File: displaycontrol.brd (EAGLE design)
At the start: 77.6 x 58.7 mm, 49 parts, among them IC1 25LC080SN, J1 GRPB052VWQS-RC, J2 5.5x2.1mm Barrel, J3 98424-F52, Q1 MMPQ3904, U1 LPC1315FBD48,551, U2 ADP3300ARTZ-3.3RL7, U3 UDN2987LWTR-6-T, U4 UDN2987LWTR-6-T, Y1 12MHz

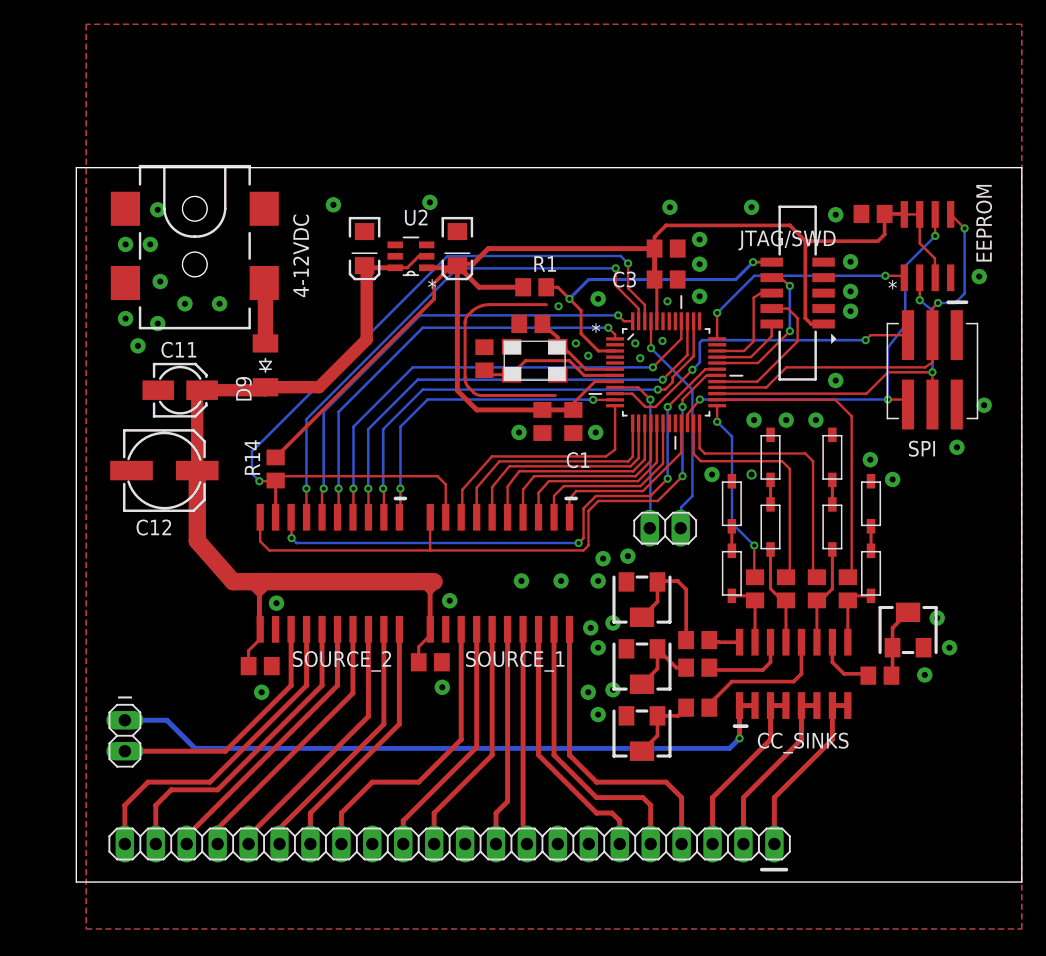
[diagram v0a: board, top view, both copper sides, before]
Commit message: changed trans
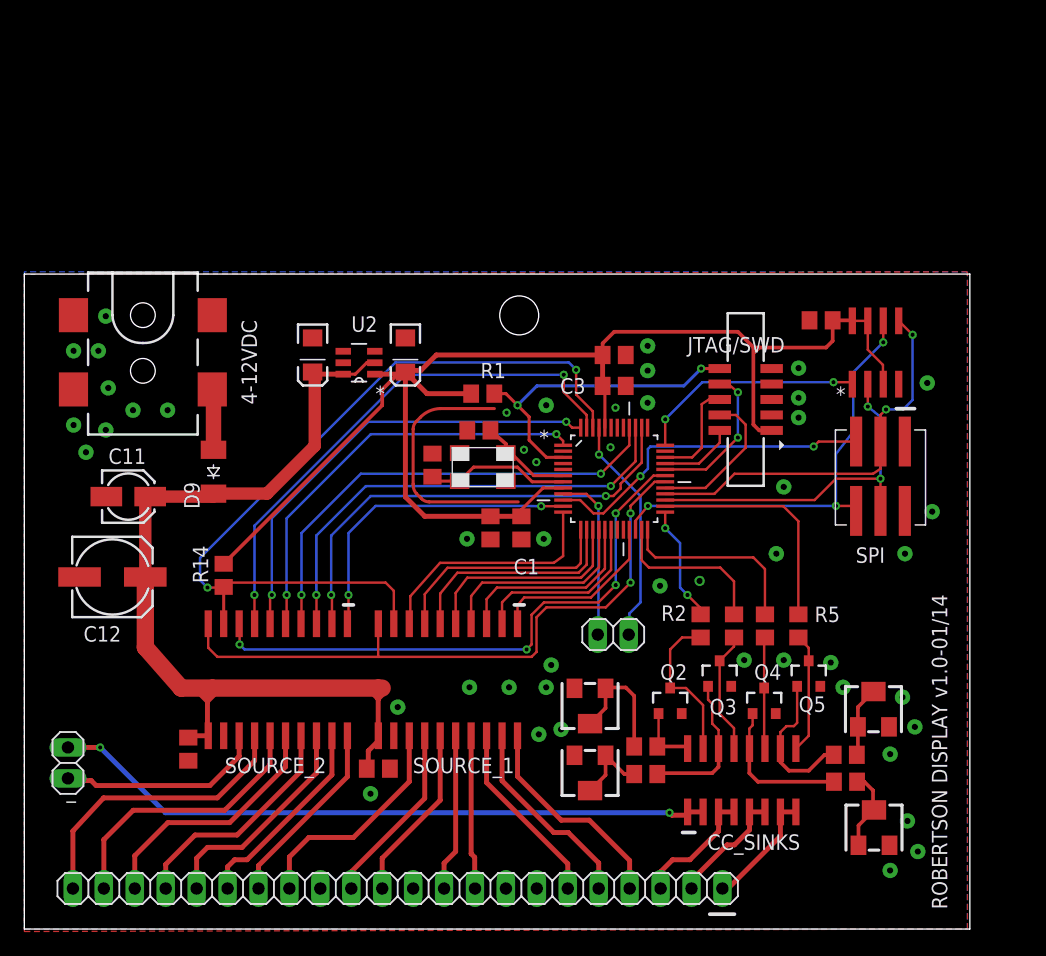
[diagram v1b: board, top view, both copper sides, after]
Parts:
- removed D1, D2, D3, D4, D5, D6, D7, D8: MMSD4148, adafruit:SOD-123
- added Q2, Q3, Q4, Q5: MMBT3904, SparkFun-DiscreteSemi:SOT23-3
- R2, R3, R4, R5: value 4.7k -> 2.7k
- R6, R7, R8, R9: value 14 -> 10
- moved R11 20.6 mm to (69.8, 8.33), turned to 0 degrees
- moved R8 13.6 mm to (67.4, 12.1), turned to 0 degrees
- moved C5 9.72 mm to (37.3, 41.0)
- moved C7 9.72 mm to (23.7, 47.1)
- moved C8 9.72 mm to (31.3, 47.1)
- moved IC1 9.72 mm to (69.9, 47.3)
- moved J3 9.72 mm to (70.3, 37.2)
- moved R6 9.72 mm to (51.0, 15.0)
- moved R7 9.72 mm to (51.0, 12.7)
- moved U4 9.72 mm to (34.8, 20.5)
- moved C11 9.72 mm to (8.53, 35.5)
- moved J2 9.72 mm to (9.73, 50.4)
- moved R14 9.72 mm to (16.4, 29.0)
- moved U2 9.72 mm to (27.5, 46.5)
- moved U3 9.72 mm to (20.8, 20.5)
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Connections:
- removed net N$10: Q1.16, R6.1
- removed net N$11: D5.A, Q1.11, R4.2
- removed net N$12: D5.C, D6.A
- removed net N$14: D7.A, Q1.9, R5.2
- removed net N$15: D7.C, D8.A
- removed net N$17: Q1.14, R7.1
- removed net N$19: Q1.12, R8.1
- removed net N$21: Q1.10, R9.1
- removed net N$5: D1.A, Q1.15, R2.2
- removed net N$8: D3.A, Q1.13, R3.2
- removed net N$9: D3.C, D4.A
- new net COLCTRL_1: Q1.9, Q5.3, R5.2
- new net COLCTRL_2: Q1.11, Q4.3, R4.2
- new net COLCTRL_3: Q1.13, Q3.3, R3.2
- new net COLCTRL_A: Q1.15, Q2.3, R2.2
- new net EMITCTRL_1: Q1.10, Q5.1, R9.1
- new net EMITCTRL_2: Q1.12, Q4.1, R8.1
- new net EMITCTRL_3: Q1.14, Q3.1, R7.1
- new net EMITCTRL_A: Q1.16, Q2.1, R6.1
- net GND: now also Q2.2, Q3.2, Q4.2, Q5.2; no longer D2.C, D4.C, D6.C, D8.C
- net N$6: now also U1.42; no longer D1.C, D2.A
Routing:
- net COLCTRL_A: track 0.00 -> 12.9 mm
- net EMITCTRL_1: track 0.00 -> 12.4 mm
- net EMITCTRL_2: track 0.00 -> 12.3 mm
- net EMITCTRL_3: track 0.00 -> 12.2 mm
- net N$19: track 11.5 -> 0.00 mm
- net COLCTRL_3: track 0.00 -> 10.1 mm
- net COLCTRL_1: track 0.00 -> 9.91 mm
- net COLCTRL_2: track 0.00 -> 9.00 mm
- net N$8: track 8.33 -> 0.00 mm
- net N$11: track 8.33 -> 0.00 mm
- net SOURCE_4: track 24.8 -> 17.7 mm
- net N$17: track 7.02 -> 0.00 mm
- net SOURCE_5: track 23.1 -> 16.5 mm
- net PIN_3: track 19.9 -> 13.5 mm
- net PIN_1: track 25.0 -> 19.1 mm
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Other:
- board size 77.6 x 58.7 mm -> 77.6 x 53.8 mm
- board text added: "1"
- board text added: "2"
- board text added: "3"
- board text added: "A"
- board text added: "ROBERTSON DISPLAY v1.0-01/14"
- board text removed: "EEPROM"
